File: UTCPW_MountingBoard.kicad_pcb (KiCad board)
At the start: 2 copper layers, 38.1 x 35.6 mm, 8 parts, among them U1 UTCPW_SampleStrip

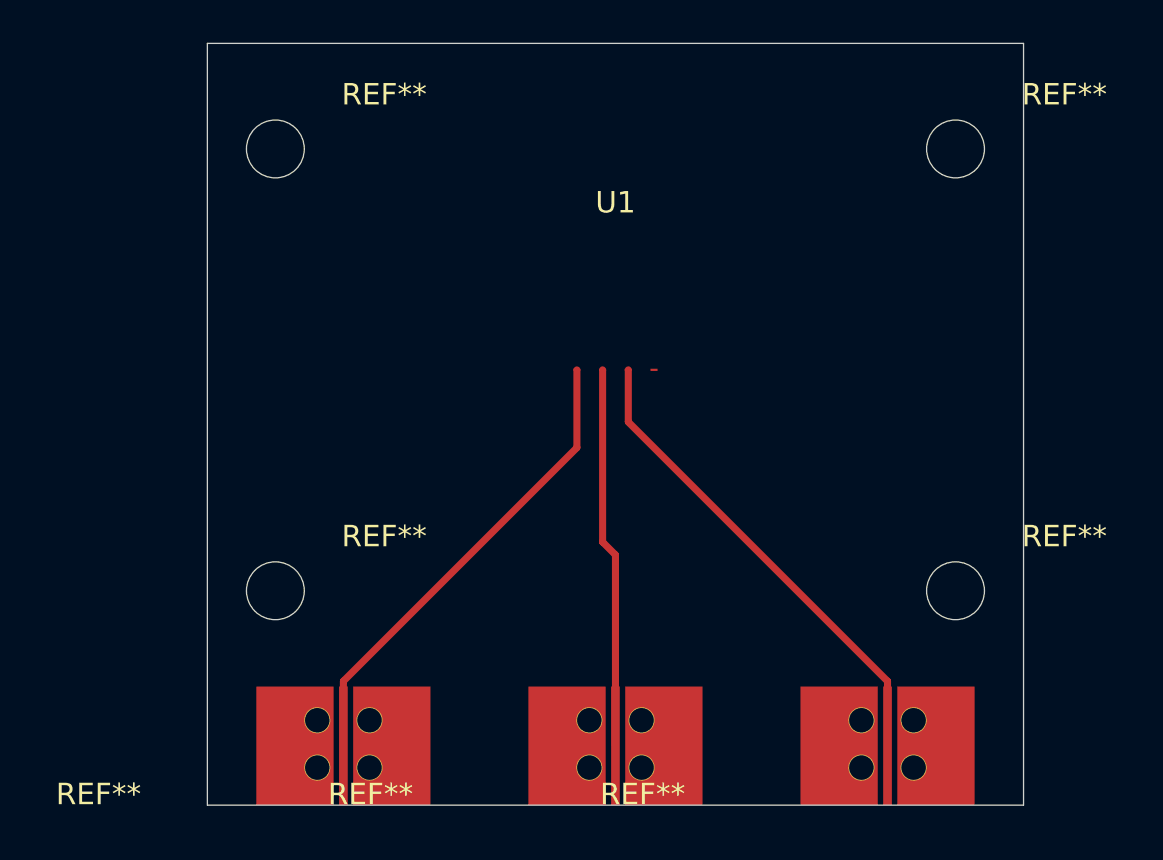
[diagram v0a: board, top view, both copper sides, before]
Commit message: Updated Gerber
Initial version for the new board
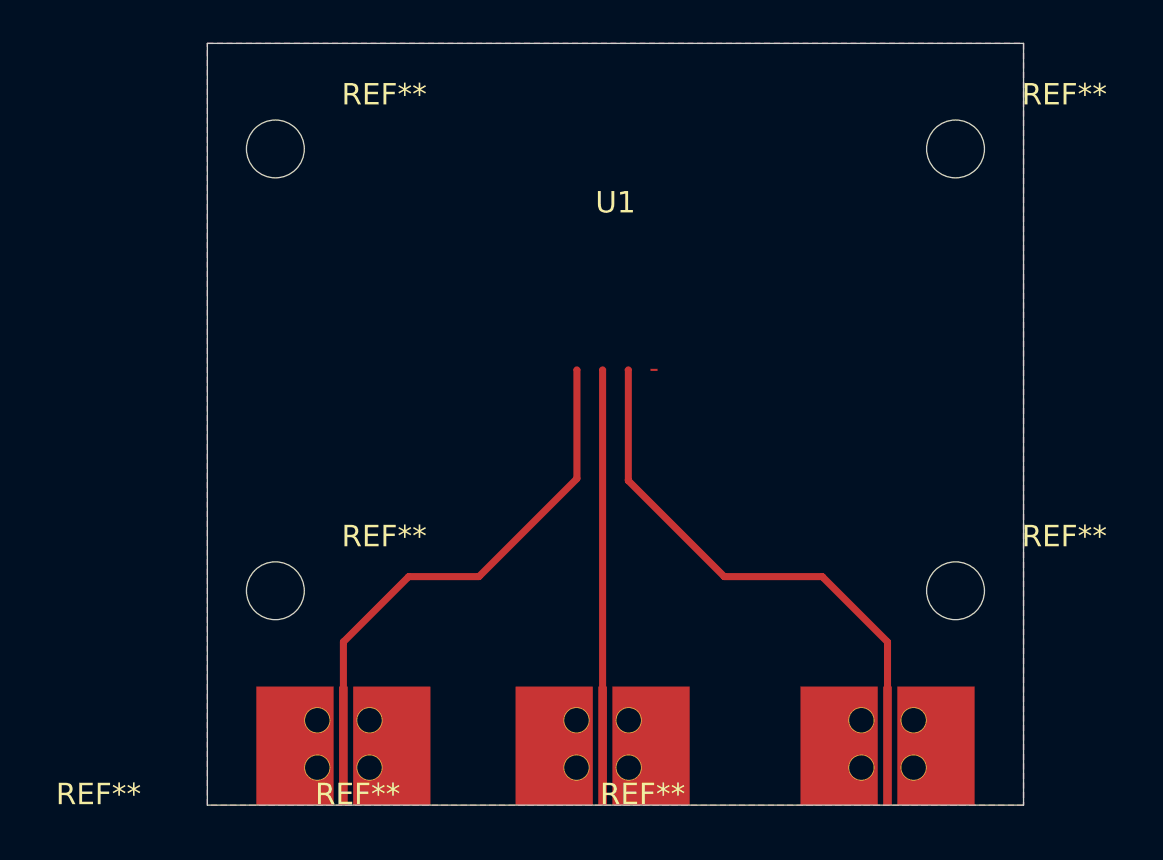
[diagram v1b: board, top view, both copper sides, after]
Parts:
- moved REF** 0.60 mm to (126.4, 121.9)
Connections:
- REF** pad 2: (no net) -> /GND (x2)
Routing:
- net /Dev3: track 22.6 -> 25.2 mm
- net /Dev1: track 22.1 -> 24.0 mm
- added copper zone on B.Cu, net (none)
- added copper zone on F.Cu, net /GND
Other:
- net class Default removed
